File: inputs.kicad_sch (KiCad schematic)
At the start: 11 parts, among them U3 LM1815

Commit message: Boards should be placed correctly now
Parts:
- D2: JLCPCB C126319 -> C84263
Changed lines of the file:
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@@
       (effects (font (size 1.27 1.27)) hide)
     )
-    (property "JLCPCB" "C126319" (id 4) (at 254 50.8 90)
+    (property "JLCPCB" "C84263" (id 4) (at 254 50.8 90)
       (effects (font (size 1.27 1.27)) hide)
     )

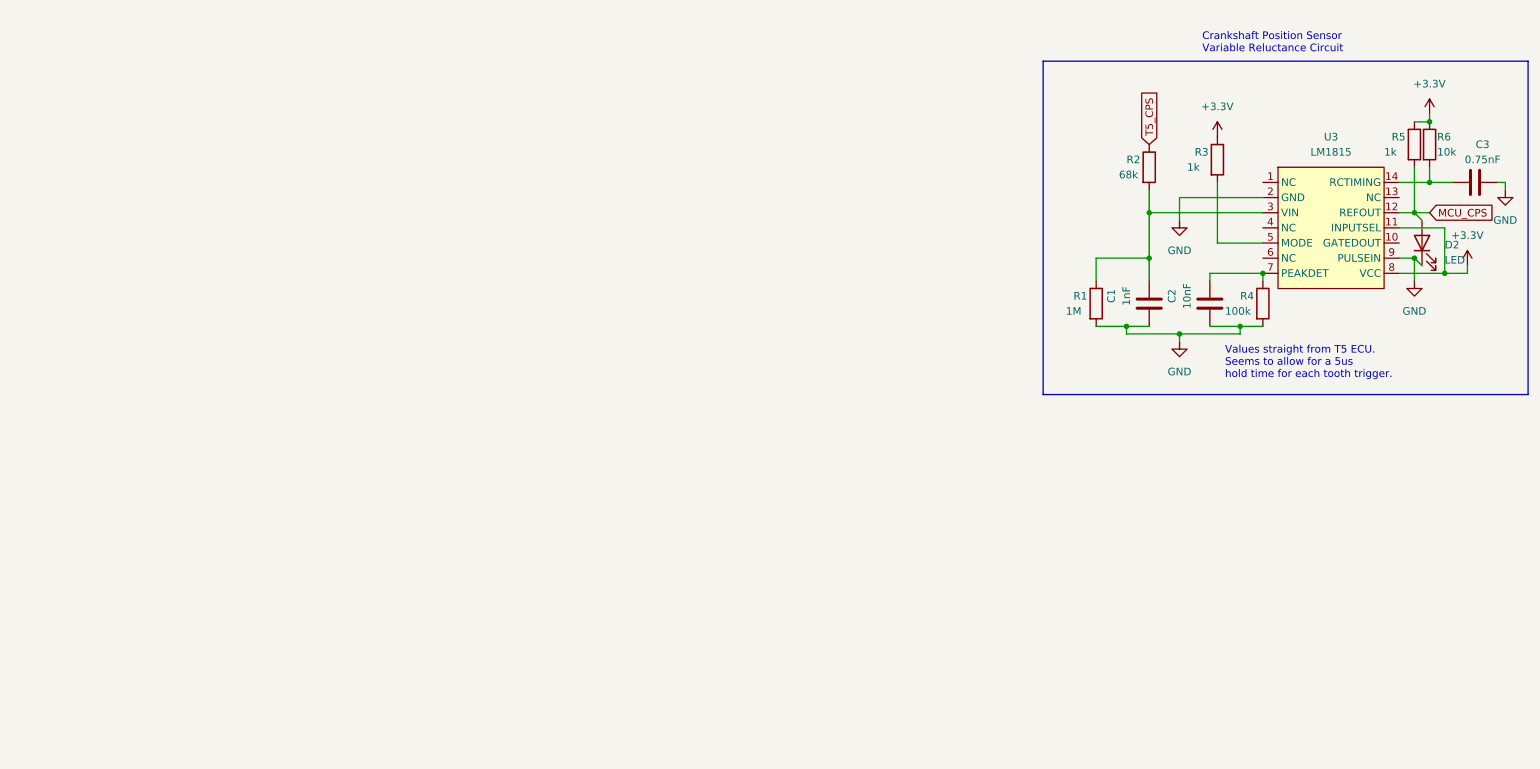
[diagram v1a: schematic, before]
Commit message: Add JLCPCB Components
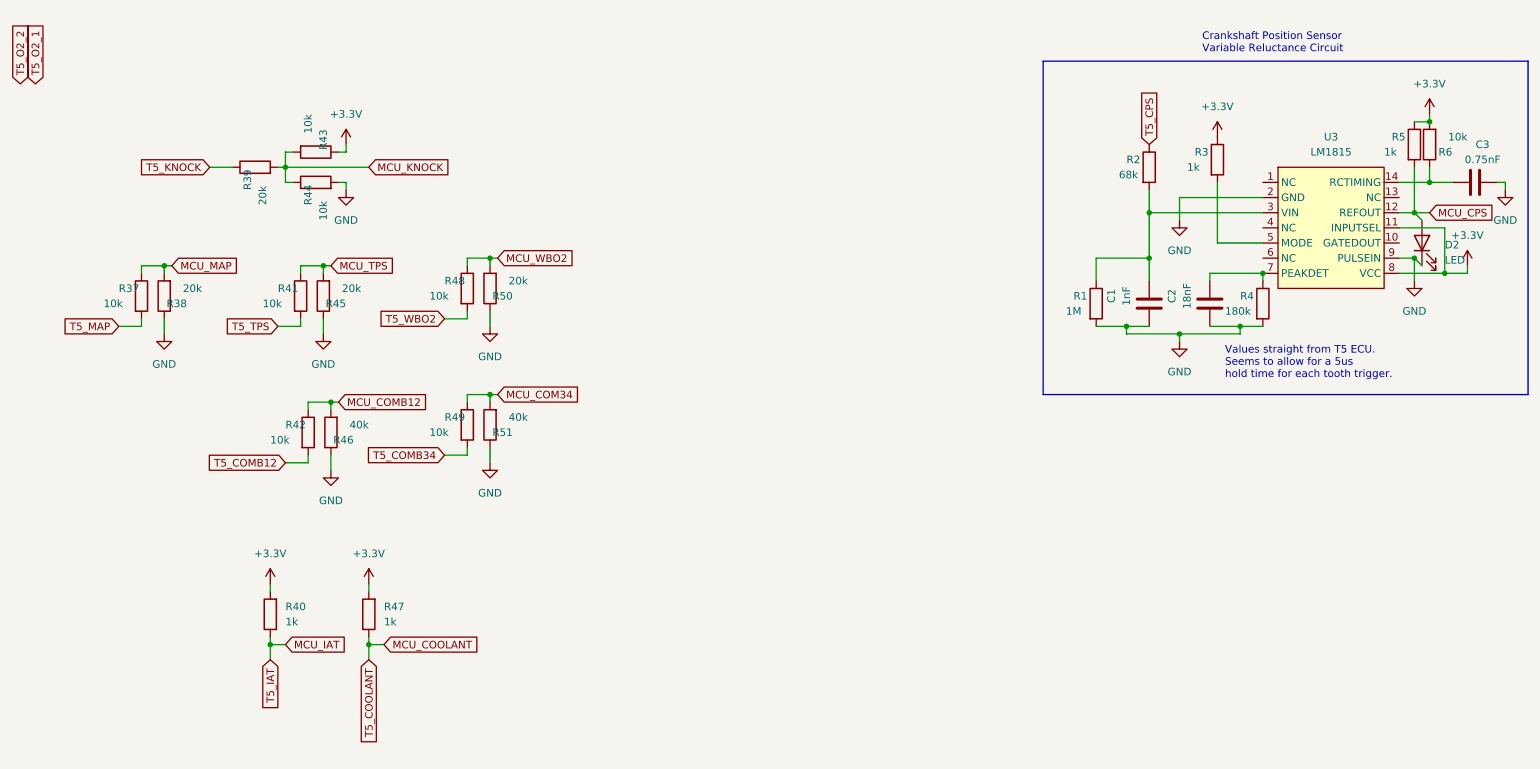
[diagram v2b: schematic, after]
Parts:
- added R37, R41, R42, R43, R44, R48, R49: 10k, Resistor_SMD:R_0603_1608Metric, symbol Device:R
- added R38, R39, R45, R50: 20k, Resistor_SMD:R_0603_1608Metric, symbol Device:R
- added R40, R47: 1k, Resistor_SMD:R_0603_1608Metric, symbol Device:R
- added R46, R51: 40k, Resistor_SMD:R_0603_1608Metric, symbol Device:R
- C1: JLCPCB (none) -> C296015
- C2: value 10nF -> 18nF; JLCPCB (none) -> C424843
- C3: JLCPCB (none) -> C576855
- R1: JLCPCB (none) -> C188125
- R2: JLCPCB (none) -> C2933251
- R4: value 100k -> 180k; JLCPCB (none) -> C100822
- R6: JLCPCB (none) -> C21190
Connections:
- net +3.3V: now also R6.2, R40.2, R43.1, R47.2; no longer R6.1
- net GND: now also R38.1, R44.2, R45.1, R46.1, R50.1, R51.1
- net at C3.1, U3.14 (RCTIMING): now also R6.1; no longer R6.2
- new net MCU_COM34: R49.1, R51.2
- new net MCU_COMB12: R42.1, R46.2
- new net MCU_COOLANT: R47.1
- new net MCU_IAT: R40.1
- new net MCU_KNOCK: R39.2, R43.2, R44.1
- new net MCU_MAP: R37.1, R38.2
- new net MCU_TPS: R41.1, R45.2
- new net MCU_WBO2: R48.1, R50.2
- new net T5_COMB12: R42.2
- new net T5_COMB34: R49.2
- new net T5_KNOCK: R39.1
- new net T5_MAP: R37.2
- new net T5_TPS: R41.2
- new net T5_WBO2: R48.2

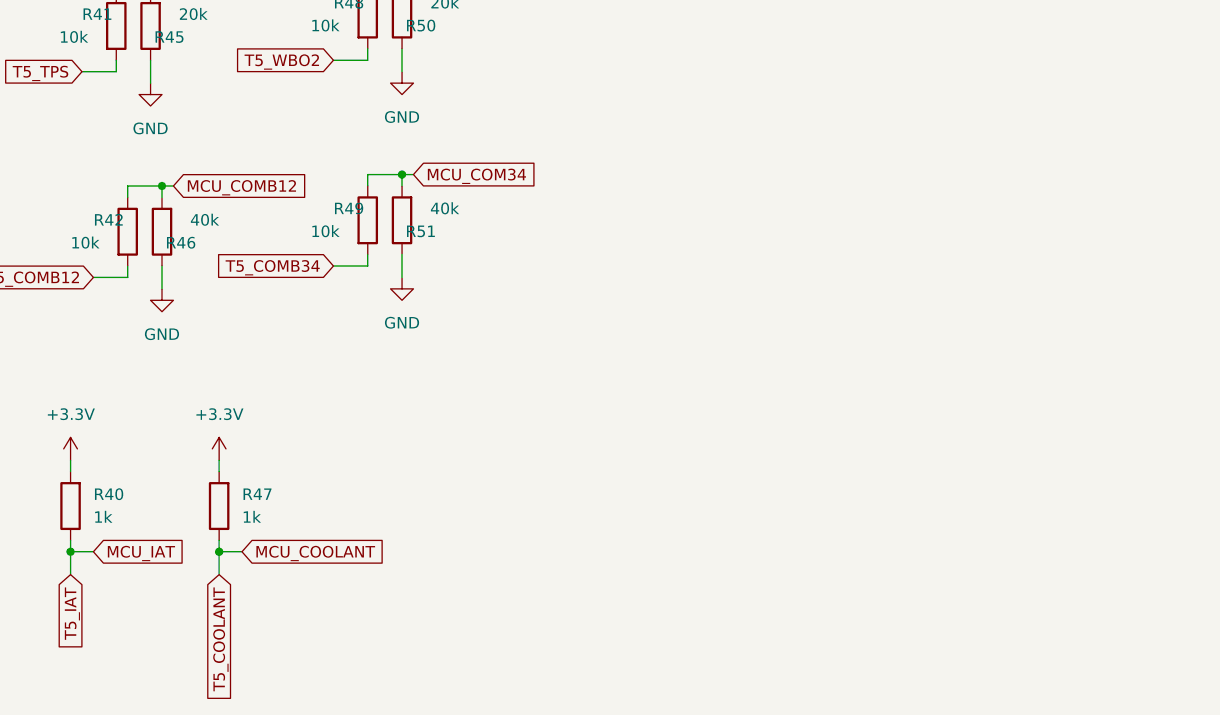
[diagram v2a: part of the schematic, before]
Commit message: More changes
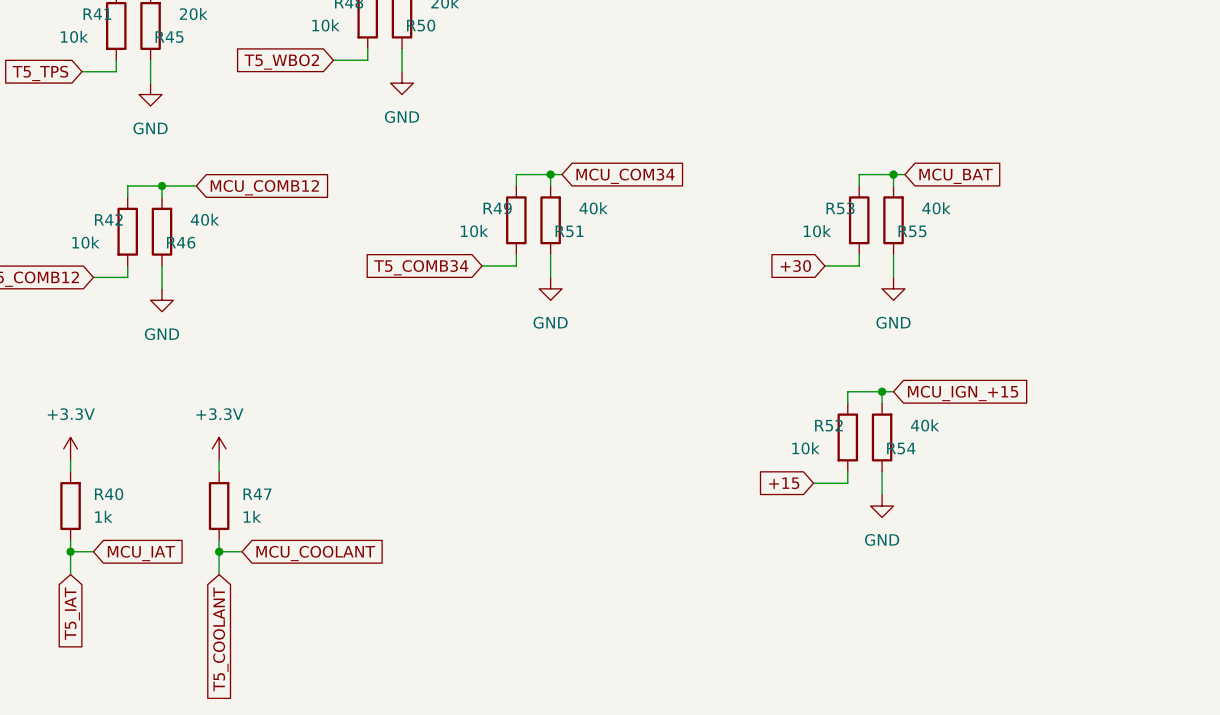
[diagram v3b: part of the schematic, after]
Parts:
- added R52, R53: 10k, Resistor_SMD:R_0603_1608Metric, symbol Device:R
- added R54, R55: 40k, Resistor_SMD:R_0603_1608Metric, symbol Device:R
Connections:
- net GND: now also R54.1, R55.1
- new net +15: R52.2
- new net +30: R53.2
- new net MCU_BAT: R53.1, R55.2
- new net MCU_IGN_+15: R52.1, R54.2
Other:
- moved on the sheet: R49, R51
